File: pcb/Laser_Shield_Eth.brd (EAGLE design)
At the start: 68.6 x 53.3 mm, 68 parts, among them IC1 CAT811TTBI-CT3, IC11 74LVC1G14DBV, IC2 MC33269ST-3, IC3 MC33269D-3, IC4 W5100, J4 JUMPER_SOLDER_1X2, J5 JUMPER_SOLDER_1X2, J6 JUMPER_SOLDER_1X2, Q1 25MHz, Q2 MOSFET-NCHANNELSMD, U1 SN74LVC2G241DCUT

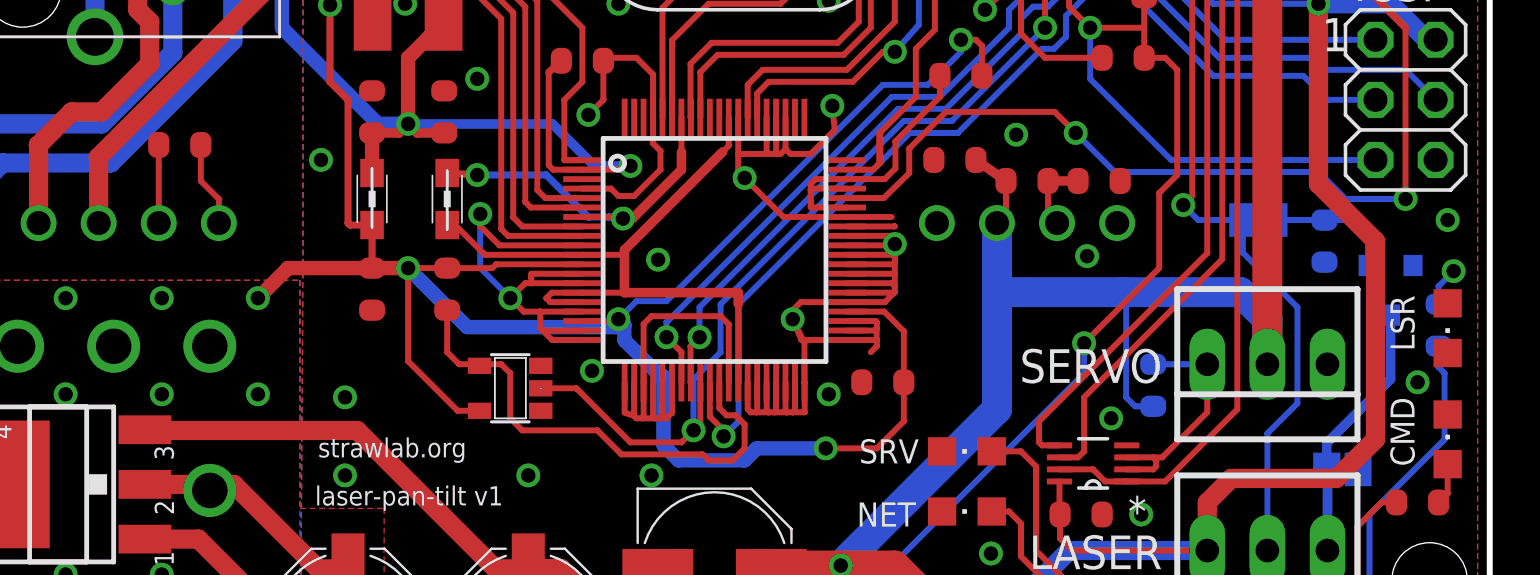
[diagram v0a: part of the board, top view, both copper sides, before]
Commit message: final pcb airwires tidy
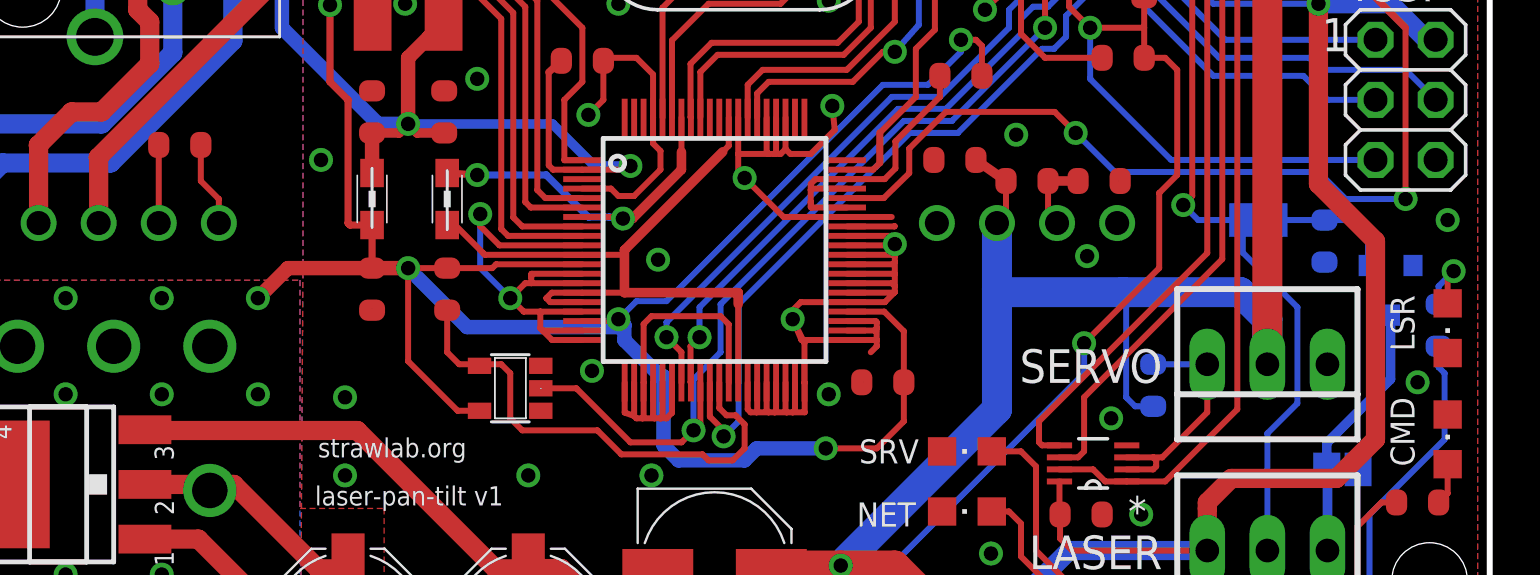
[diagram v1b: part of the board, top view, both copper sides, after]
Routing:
- net N$5: track 1.66 -> 3.13 mm
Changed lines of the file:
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@@
 <layer number="49" name="Reference" color="13" fill="1" visible="no" active="yes"/>
 <layer number="50" name="dxf" color="12" fill="1" visible="no" active="yes"/>
-<layer number="51" name="tDocu" color="7" fill="1" visible="yes" active="yes"/>
+<layer number="51" name="tDocu" color="7" fill="1" visible="no" active="yes"/>
 <layer number="52" name="bDocu" color="7" fill="1" visible="no" active="yes"/>
 <layer number="91" name="Nets" color="2" fill="1" visible="no" active="no"/>
@@
 <wire x1="50.419" y1="9.398" x2="50.927" y2="8.89" width="0.254" layer="1"/>
 <wire x1="50.927" y1="8.89" x2="56.642" y2="8.89" width="0.254" layer="1"/>
-<wire x1="11.912" y1="13.964" x2="11.7348" y2="13.9954" width="0" layer="19" extent="1-1"/>
+<wire x1="11.7348" y1="13.9954" x2="11.8806" y2="13.9954" width="0.254" layer="1"/>
+<wire x1="11.8806" y1="13.9954" x2="11.912" y2="13.964" width="0.254" layer="1"/>
 </signal>
 <signal name="GND" class="1">
@@
 <signal name="N$32">
 <contactref element="R6" pad="1"/>
-<wire x1="12.319" y1="25.146" x2="12.319" y2="26.035" width="0.254" layer="1"/>
 <via x="12.319" y="22.733" extent="1-16" drill="1.016" shape="octagon"/>
-<wire x1="12.319" y1="25.1212" x2="12.319" y2="22.733" width="0.254" layer="1"/>
-<wire x1="12.319" y1="25.1212" x2="12.319" y2="25.146" width="0" layer="19" extent="1-1"/>
+<wire x1="12.319" y1="26.035" x2="12.319" y2="22.733" width="0.254" layer="1"/>
 </signal>
 <signal name="N$33">
@@
 <wire x1="66.421" y1="20.066" x2="67.056" y2="20.701" width="0.254" layer="16"/>
 <via x="67.056" y="20.701" extent="1-16" drill="0.6096" shape="octagon"/>
-<wire x1="66.421" y1="19.304" x2="66.802" y2="19.338" width="0" layer="19" extent="1-16"/>
+<wire x1="66.802" y1="19.338" x2="66.802" y2="20.447" width="0.254" layer="1"/>
+<wire x1="66.802" y1="20.447" x2="67.056" y2="20.701" width="0.254" layer="1"/>
 </signal>
 <signal name="N$11">
